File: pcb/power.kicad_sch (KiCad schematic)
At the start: 15 parts, among them J4 Conn_01x02, Q1 Q_PMOS_DGS, SW1 POWER, U3 MCP73831-2-OT, U4 MAX17948, U6 MIC5353-3.3YMT

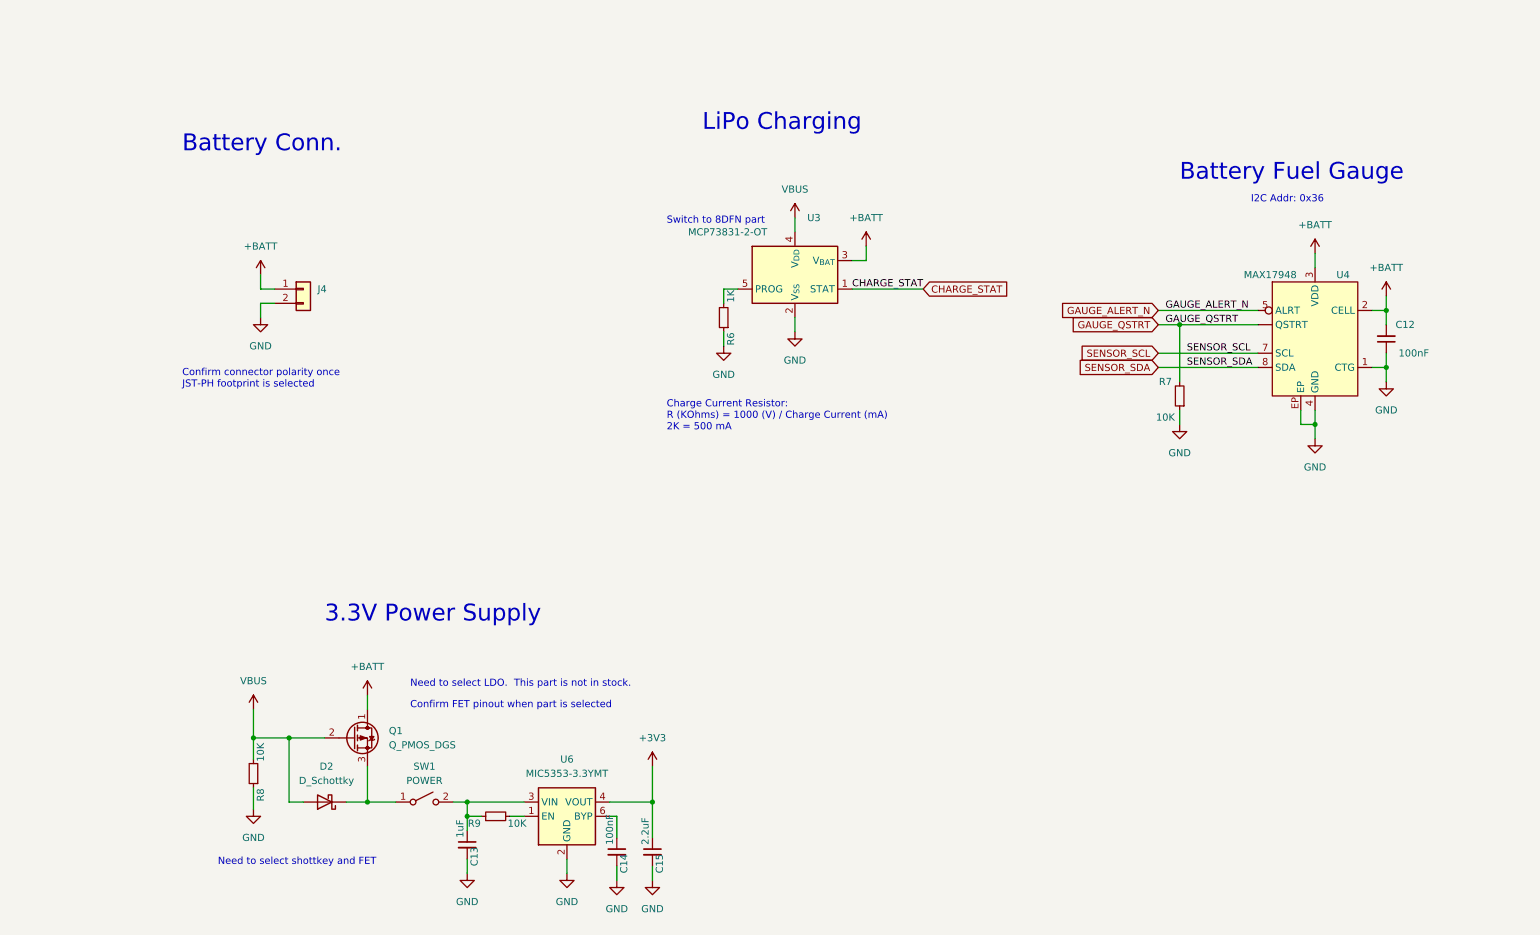
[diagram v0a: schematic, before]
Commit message: pcb: Update schematic to WIP6
Change-Id: I9e9f727ad2774ee986f2f97450dc509901129aec
Reviewed-on: https://pigweed-review.googlesource.com/c/pigweed/kudzu/+/169650
Reviewed-by: Anthony DiGirolamo <tonymd@google.com>
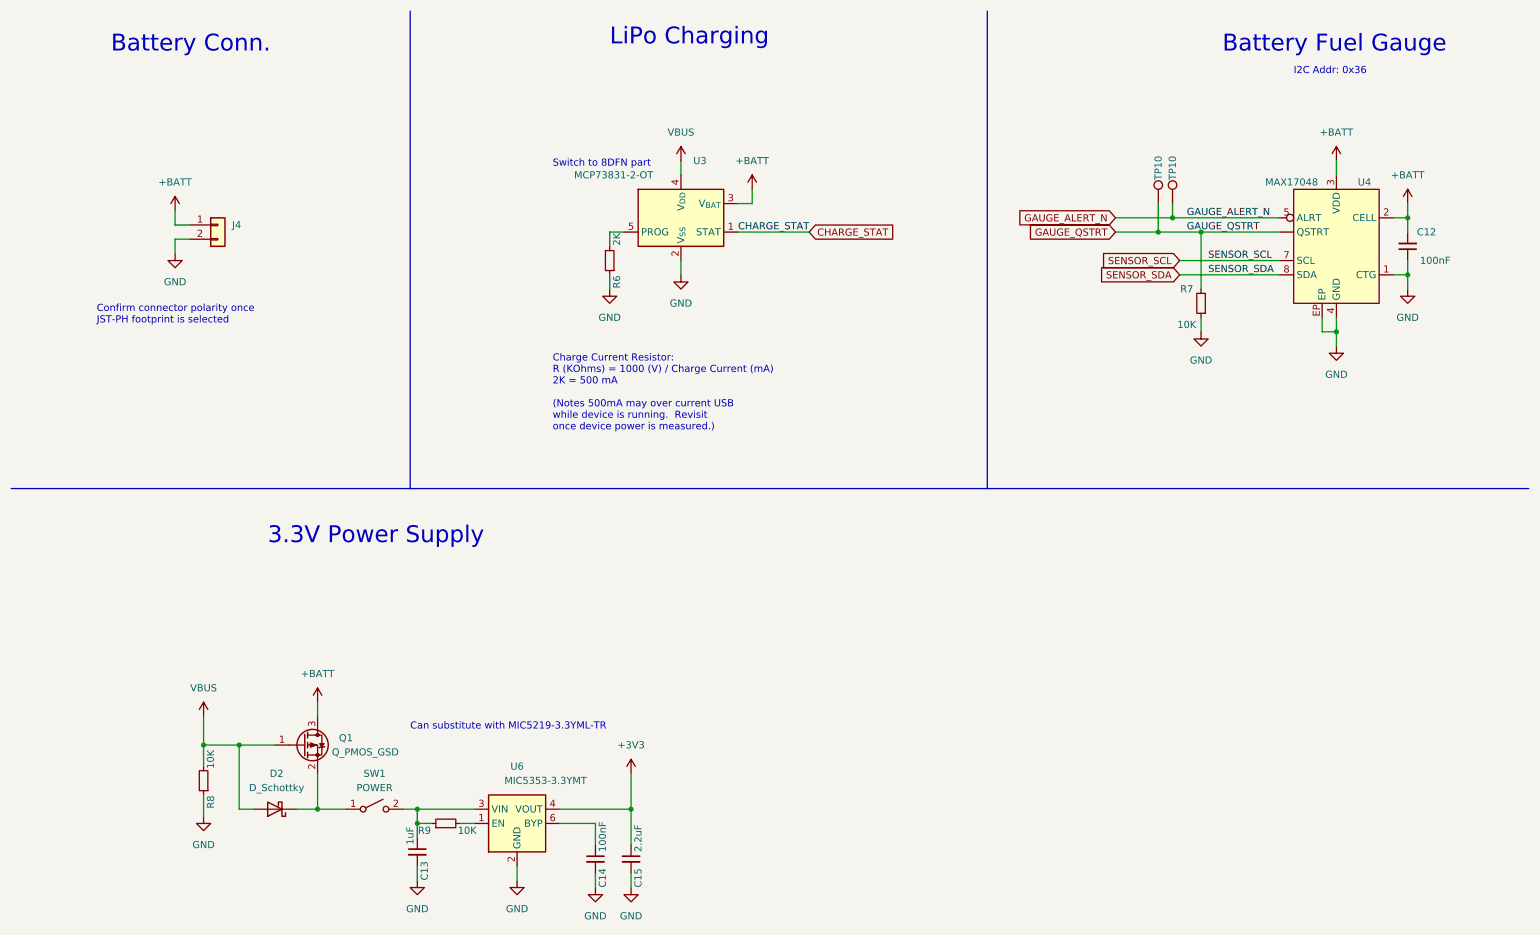
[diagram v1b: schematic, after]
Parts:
- added TP10 (x2): RUN, symbol Connector:TestPoint
- D2: DigiKey PN (none) -> 4786-B5819WCT-ND; Price @ 10 (none) -> 0.16400; Price @ 25 (none) -> 0.16400
- Q1: value Q_PMOS_DGS -> Q_PMOS_GSD; footprint (none) -> Package_TO_SOT_SMD:SOT-23-3; symbol Device:Q_PMOS_DGS -> Device:Q_PMOS_GSD; DigiKey PN (none) -> 31-DMG3415UQ-7CT-ND; Price @ 10 (none) -> 0.36000; Price @ 25 (none) -> 0.36000
- R6: value 1K -> 2K
- U3: DigiKey PN (none) -> MCP73831T-2ACI/MCTR-ND; Price @ 10 (none) -> 0.79000; Price @ 25 (none) -> 0.65000
- U4: value MAX17948 -> MAX17048; DigiKey PN (none) -> MAX17048G+T10TR-ND; Price @ 10 (none) -> 3.03900; Price @ 25 (none) -> 2.87280
- U6: DigiKey PN 76-3980-2-ND -> 576-3680-2-ND; Price @ 10 (none) -> 0.46000; Price @ 25 (none) -> 0.37000
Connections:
- net +BATT: now also Q1.3 (D); no longer Q1.1 (D)
- net GAUGE_ALERT_N: now also TP10.1
- net GAUGE_QSTRT: now also TP10.1
- net VBUS: now also Q1.1 (G); no longer Q1.2 (G)
- net at D2.1 (K), SW1.1 (A): now also Q1.2 (S); no longer Q1.3 (S)
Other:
- note added: "Can substitute with MIC5219-3.3YML-TR"
- note added: "Charge Current Resistor: R (KOhms) = 1000 (V) / Charge Current (mA) 2K = 500 mA (Notes 500mA may over current USB while device is running. Revisit once device power is measured.)"
- note removed: "Charge Current Resistor: R (KOhms) = 1000 (V) / Charge Current (mA) 2K = 500 mA"
- note removed: "Confirm FET pinout when part is selected"
- note removed: "Need to select LDO. This part is not in stock."
- note removed: "Need to select shottkey and FET"
- moved on the sheet: C12, C13, C14, C15, D2, J4, Q1, R6, R7, R8, R9, SW1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
